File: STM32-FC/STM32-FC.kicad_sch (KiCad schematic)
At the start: 30 parts, among them J1 GH 1.25mm 6P, Q1 PMDPB30XN, U1 STM32F407VETx, Y1 16MHz

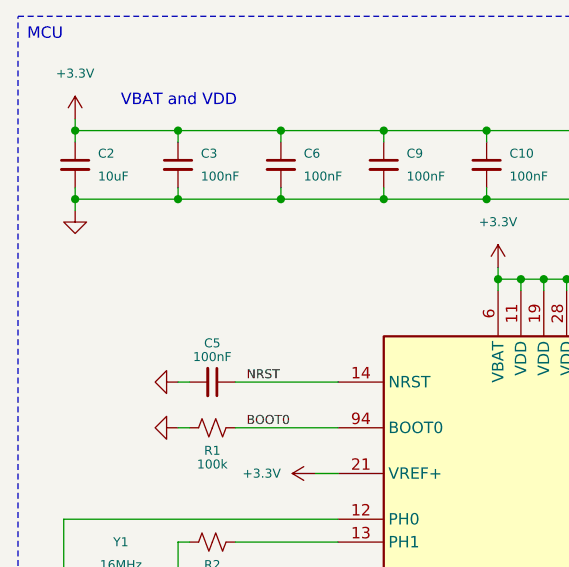
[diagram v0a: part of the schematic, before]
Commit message: update : Development board
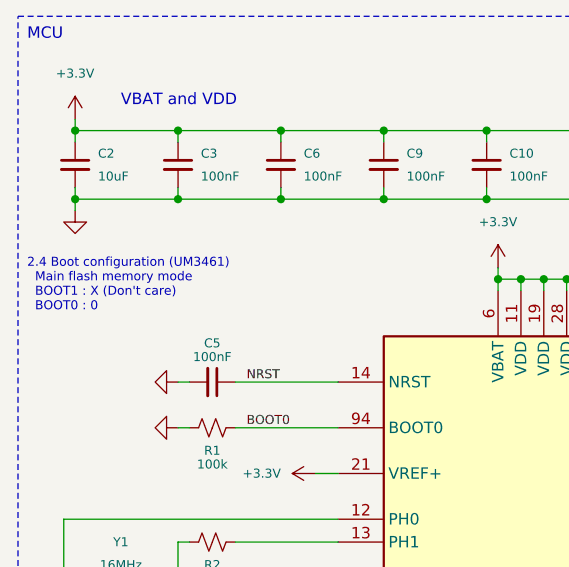
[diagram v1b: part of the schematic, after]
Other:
- note added: "2.4 Boot configuration (UM3461) Main flash memory mode BOOT1 : X (Don't care) BOOT0 : 0"
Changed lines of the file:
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@@
+		)
+	)
+	(text "2.4 Boot configuration (UM3461)\n  Main flash memory mode\n  BOOT1 : X (Don't care)\n  BOOT0 : 0\n"
+		(exclude_from_sim no)
+		(at 25.146 40.894 0)
+		(effects
+			(font
+				(size 1 1)
+			)
+			(justify left top)
 		)
 	)
